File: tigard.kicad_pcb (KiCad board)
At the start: 4 copper layers, 46 x 46 mm, 94 parts, among them J1 USB_C_Receptacle_USB2.0, J2 JTAG, J3 UART, J4 SPI, J5 CORTEX, J6 LA, J7 I2C, J8 CORTEX, J9 LA, Q1 BSH103, SW1 TARGET, SW2 MODE, U1 AP7365-18, U2 AP7365-33, U3 FT2232HQ, U4 93LC46BT-I/OT, U5 SN74LVC8T245, U6 SN74LVC8T245, Y1 12MHz

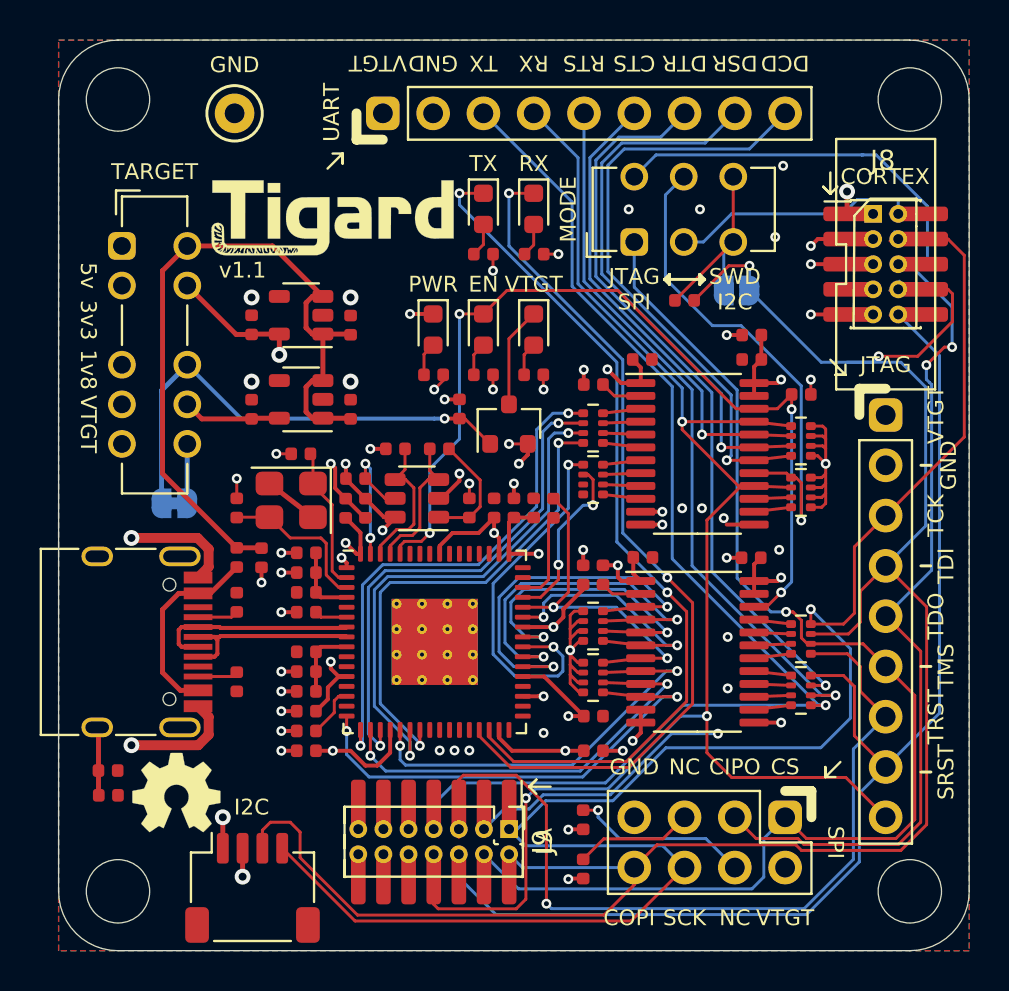
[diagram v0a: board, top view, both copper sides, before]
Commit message: v.2.2
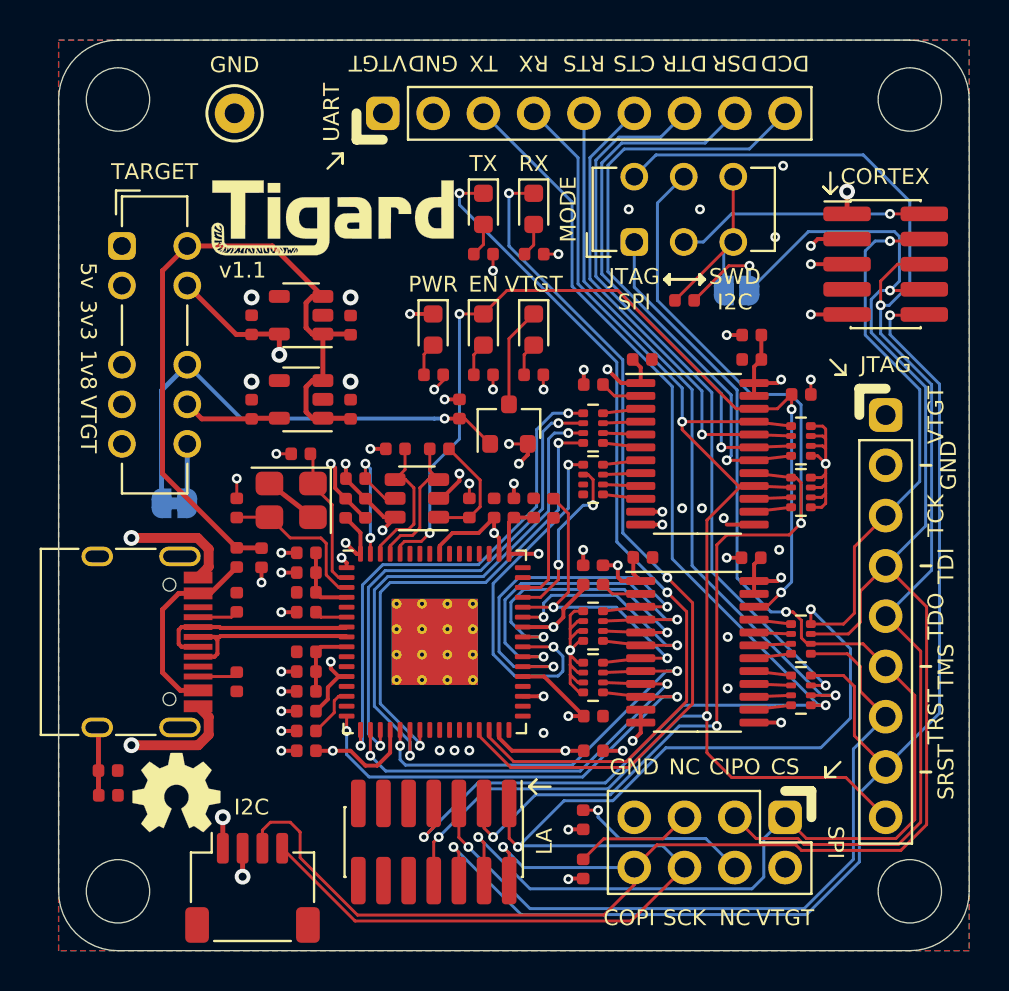
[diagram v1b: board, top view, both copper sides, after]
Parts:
- removed J8: CORTEX, mybays_connector:debugger_2x05_P1.27mm_Vertical
- removed J9: LA, Connector_PinHeader_1.27mm:PinHeader_2x07_P1.27mm_Vertical
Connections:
- J1 pad A8: Net-(J1-PadA8) -> (no net)
- J1 pad B8: Net-(J1-PadB8) -> (no net)
- J5 pad 7: Net-(J5-Pad7) -> (no net)
- J6 pad 11: Net-(J6-Pad11) -> (no net)
- J6 pad 12: Net-(J6-Pad12) -> (no net)
- J6 pad 13: Net-(J6-Pad13) -> (no net)
- J6 pad 14: Net-(J6-Pad14) -> (no net)
- RN6 pad 3: Net-(RN6-Pad3) -> (no net)
- RN6 pad 4: Net-(RN6-Pad4) -> (no net)
- SW1 pad 1: Net-(SW1-Pad1) -> (no net)
- SW1 pad 2: Net-(SW1-Pad2) -> (no net)
- SW1 pad 3: Net-(SW1-Pad3) -> (no net)
- SW1 pad 4: Net-(SW1-Pad4) -> (no net)
- SW1 pad 5: Net-(SW1-Pad5) -> (no net)
- U1 pad 4: Net-(U1-Pad4) -> (no net)
- U2 pad 4: Net-(U2-Pad4) -> (no net)
- U3 pad 24: Net-(U3-Pad24) -> (no net)
- U3 pad 26: Net-(U3-Pad26) -> (no net)
- U3 pad 27: Net-(U3-Pad27) -> (no net)
- U3 pad 28: Net-(U3-Pad28) -> (no net)
- U3 pad 32: Net-(U3-Pad32) -> (no net)
- U3 pad 33: Net-(U3-Pad33) -> (no net)
- U3 pad 34: Net-(U3-Pad34) -> (no net)
- U3 pad 36: Net-(U3-Pad36) -> (no net)
- U3 pad 48: Net-(U3-Pad48) -> (no net)
- U3 pad 52: Net-(U3-Pad52) -> (no net)
- U3 pad 53: Net-(U3-Pad53) -> (no net)
- U3 pad 54: Net-(U3-Pad54) -> (no net)
- U3 pad 55: Net-(U3-Pad55) -> (no net)
- U3 pad 57: Net-(U3-Pad57) -> (no net)
- U3 pad 58: Net-(U3-Pad58) -> (no net)
- U3 pad 59: Net-(U3-Pad59) -> (no net)
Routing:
- net /xPB4: track 44.7 -> 37.9 mm
- net GND: track 57.0 -> 50.4 mm
- net /ICE_CDONE: track 80.0 -> 74.9 mm
- net /COPI: track 108.5 -> 104.5 mm, vias 2 -> 3
- net /CORTEX_PIN2: track 15.5 -> 12.7 mm, vias 0 -> 1
- net /DI: track 53.8 -> 56.2 mm, vias 2 -> 3
- net /xPB5: track 66.5 -> 64.2 mm, vias 0 -> 2
- net /CLK: track 89.2 -> 87.3 mm, vias 1 -> 3
- net /CS: track 64.6 -> 66.3 mm, vias 1 -> 2
- net VTARGET: track 130.6 -> 129.2 mm
- net /CIPO: track 65.4 -> 64.5 mm, vias 2 -> 1
- net /UART_TX: track 63.6 -> 63.0 mm, vias 1 -> 2

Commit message: rev1
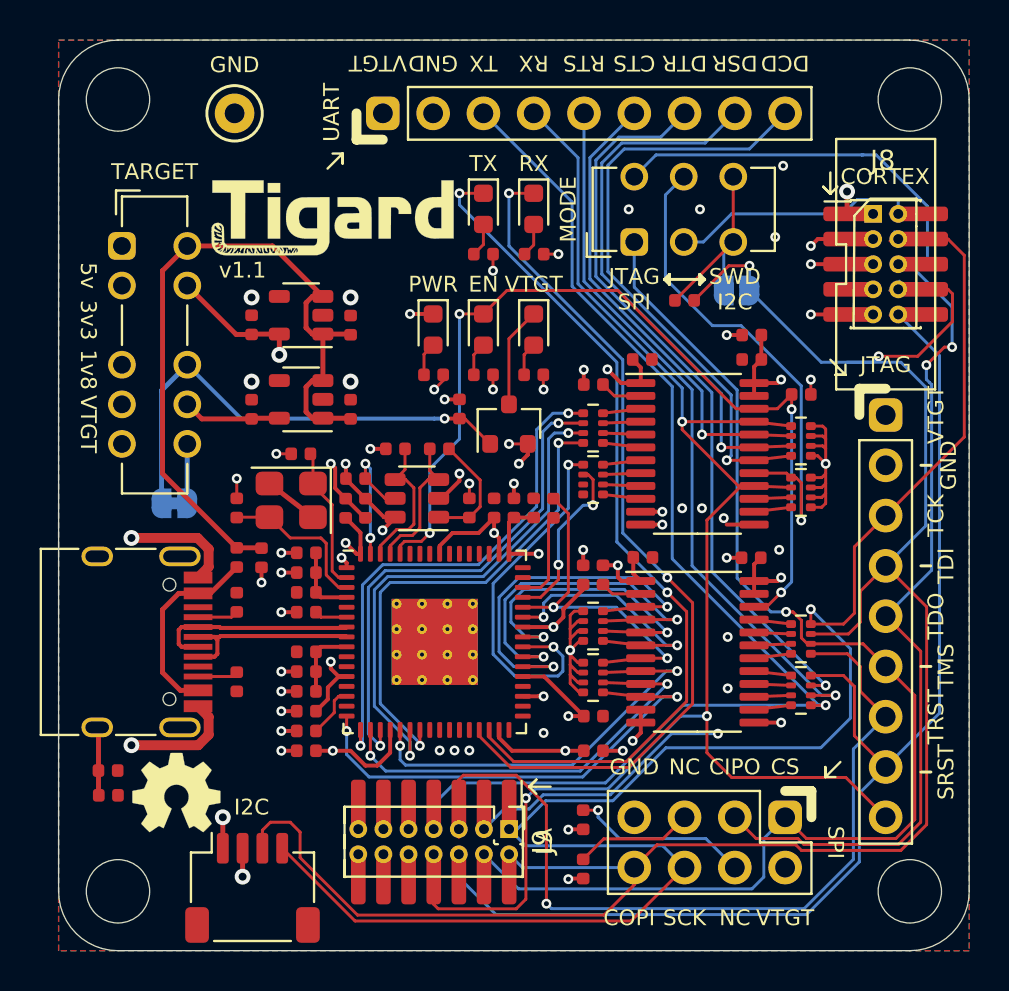
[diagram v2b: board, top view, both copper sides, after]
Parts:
- added J8: CORTEX, mybays_connector:debugger_2x05_P1.27mm_Vertical, F.Cu at (71.8, 41.3)
- added J9: LA, Connector_PinHeader_1.27mm:PinHeader_2x07_P1.27mm_Vertical, F.Cu at (52.8, 69.9)
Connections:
- J1 pad A8: (no net) -> Net-(J1-PadA8)
- J1 pad B8: (no net) -> Net-(J1-PadB8)
- J5 pad 7: (no net) -> Net-(J5-Pad7)
- J6 pad 11: (no net) -> Net-(J6-Pad11)
- J6 pad 12: (no net) -> Net-(J6-Pad12)
- J6 pad 13: (no net) -> Net-(J6-Pad13)
- J6 pad 14: (no net) -> Net-(J6-Pad14)
- RN6 pad 3: (no net) -> Net-(RN6-Pad3)
- RN6 pad 4: (no net) -> Net-(RN6-Pad4)
- SW1 pad 1: (no net) -> Net-(SW1-Pad1)
- SW1 pad 2: (no net) -> Net-(SW1-Pad2)
- SW1 pad 3: (no net) -> Net-(SW1-Pad3)
- SW1 pad 4: (no net) -> Net-(SW1-Pad4)
- SW1 pad 5: (no net) -> Net-(SW1-Pad5)
- U1 pad 4: (no net) -> Net-(U1-Pad4)
- U2 pad 4: (no net) -> Net-(U2-Pad4)
- U3 pad 24: (no net) -> Net-(U3-Pad24)
- U3 pad 26: (no net) -> Net-(U3-Pad26)
- U3 pad 27: (no net) -> Net-(U3-Pad27)
- U3 pad 28: (no net) -> Net-(U3-Pad28)
- U3 pad 32: (no net) -> Net-(U3-Pad32)
- U3 pad 33: (no net) -> Net-(U3-Pad33)
- U3 pad 34: (no net) -> Net-(U3-Pad34)
- U3 pad 36: (no net) -> Net-(U3-Pad36)
- U3 pad 48: (no net) -> Net-(U3-Pad48)
- U3 pad 52: (no net) -> Net-(U3-Pad52)
- U3 pad 53: (no net) -> Net-(U3-Pad53)
- U3 pad 54: (no net) -> Net-(U3-Pad54)
- U3 pad 55: (no net) -> Net-(U3-Pad55)
- U3 pad 57: (no net) -> Net-(U3-Pad57)
- U3 pad 58: (no net) -> Net-(U3-Pad58)
- U3 pad 59: (no net) -> Net-(U3-Pad59)
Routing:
- net /xPB4: track 37.9 -> 44.7 mm
- net GND: track 50.4 -> 57.0 mm
- net /ICE_CDONE: track 74.9 -> 80.0 mm
- net /COPI: track 104.5 -> 108.5 mm, vias 3 -> 2
- net /CORTEX_PIN2: track 12.7 -> 15.5 mm, vias 1 -> 0
- net /DI: track 56.2 -> 53.8 mm, vias 3 -> 2
- net /xPB5: track 64.2 -> 66.5 mm, vias 2 -> 0
- net /CLK: track 87.3 -> 89.2 mm, vias 3 -> 1
- net /CS: track 66.3 -> 64.6 mm, vias 2 -> 1
- net VTARGET: track 129.2 -> 130.6 mm
- net /CIPO: track 64.5 -> 65.4 mm, vias 1 -> 2
- net /UART_TX: track 63.0 -> 63.6 mm, vias 2 -> 1
